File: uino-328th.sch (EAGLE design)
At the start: 11 parts, among them J1 USB_MICRO_B_2.0-TH

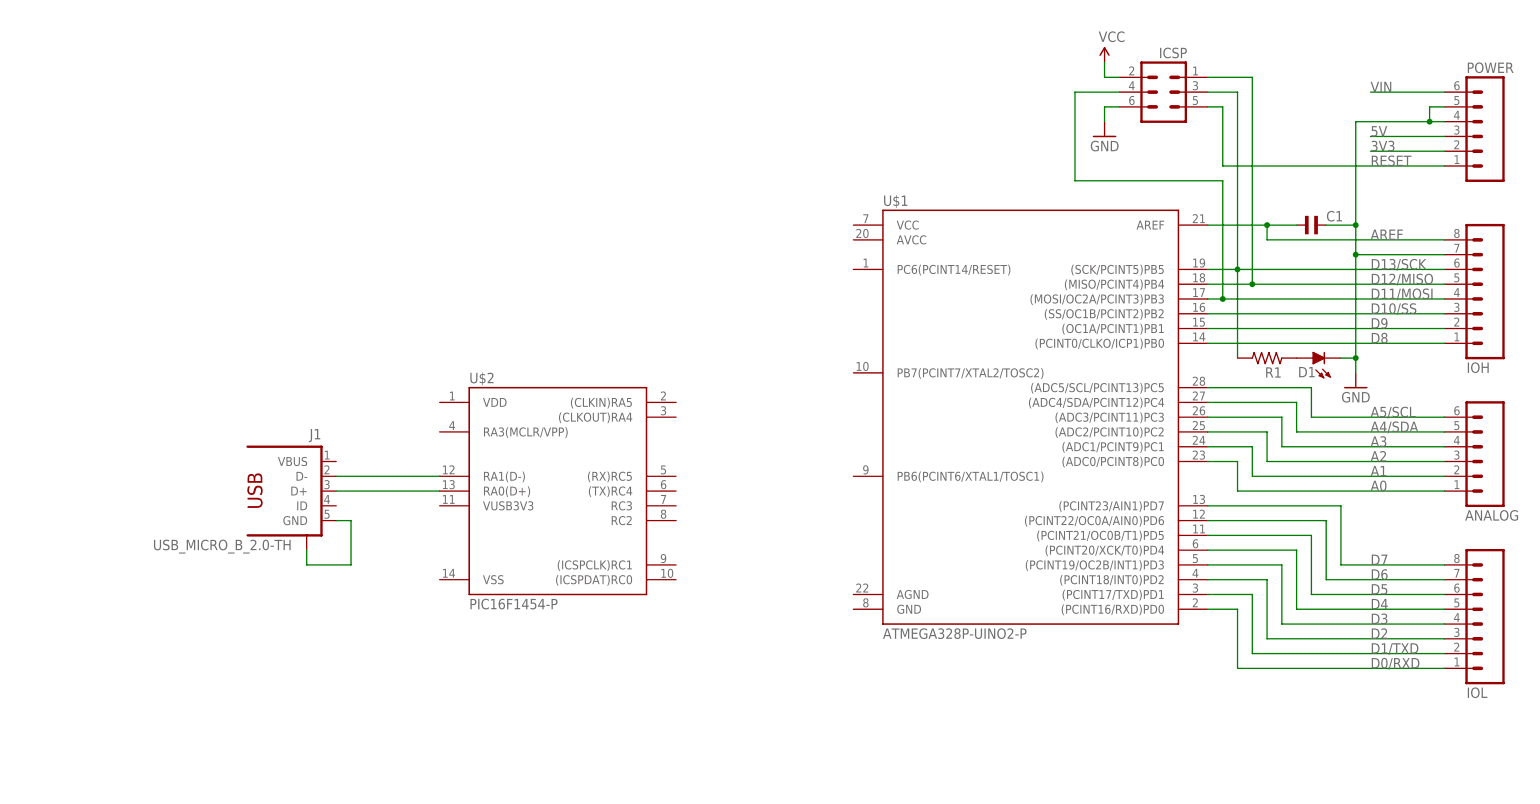
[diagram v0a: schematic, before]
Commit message: Schematic complete.
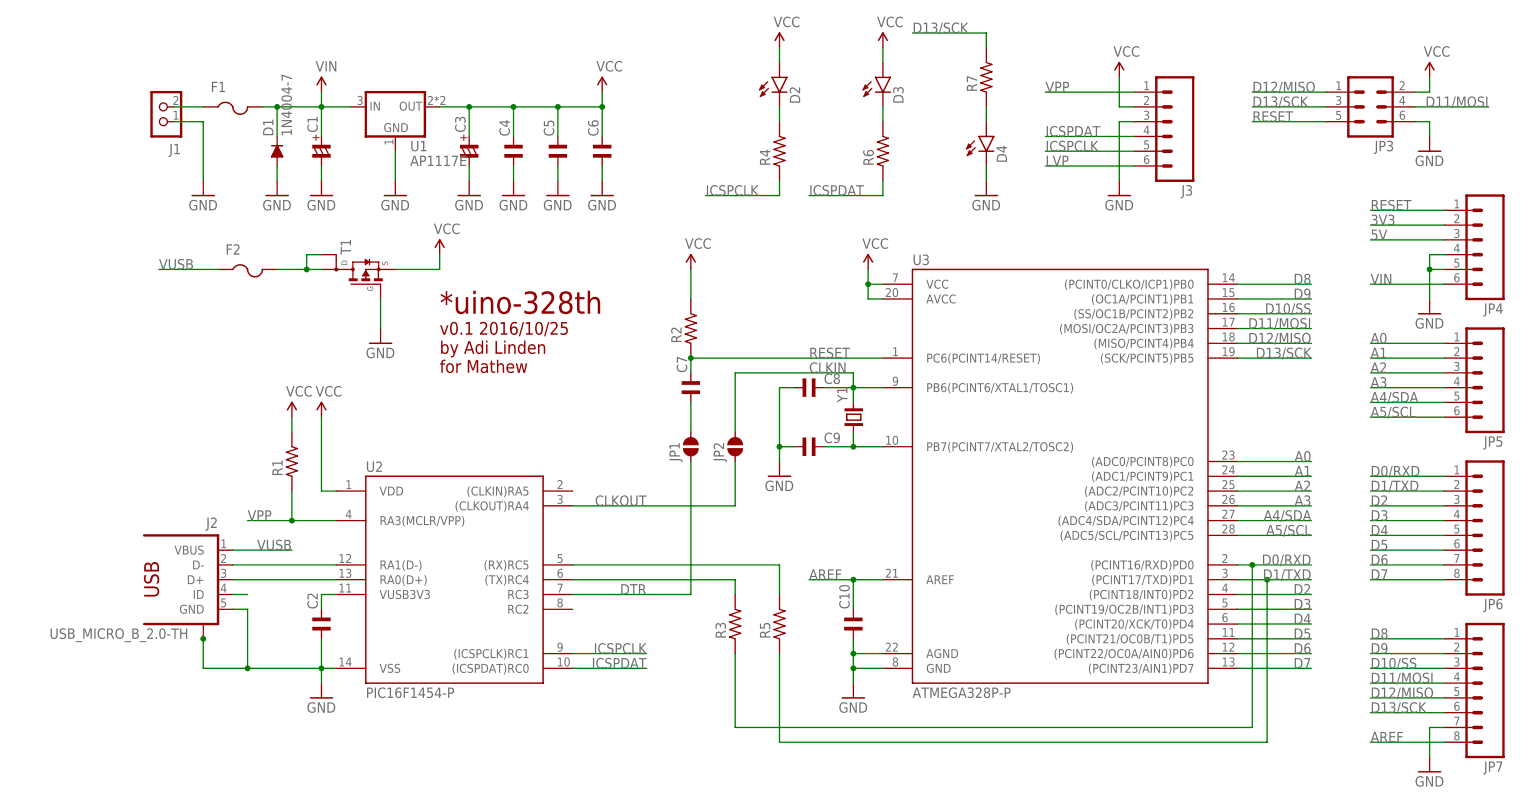
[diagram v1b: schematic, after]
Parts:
- removed ANALOG, POWER: (no value), SparkFun:M06SIP
- removed ICSP: M03X2, adilinden:M03X2
- removed IOH, IOL: (no value), SparkFun:M081X08
- removed U$1: ATMEGA328P-UINO2-P, adi-atmega:ATMEGA328P-UINO2-P
- removed U$2: PIC16F1454-P, adi-pic:PIC16F1454-P
- added C10, C2, C4, C5, C6, C7, C8, C9: (no value), rc-master-th:C_C025-040X018
- added C3: (no value), rc-master-th:CP_TT025-040
- added D2, D3, D4: (no value), SparkFun-LED:LED3MM
- added F1, F2: (no value), adi-misc:FUSE_PTC-1206
- added J2: USB_MICRO_B_2.0-TH, adi-misc:USB_MICRO_B_2.0-TH
- added J3: (no value), SparkFun-Connectors:M06LOCK
- added JP1, JP2: SJ-035, jumpers:SJ-035
- added JP3: M03X2, adi-misc:M03X2
- added JP4, JP5: (no value), SparkFun:M06SIP
- added JP6, JP7: (no value), SparkFun:M081X08
- added R2, R3, R4, R5, R6, R7: (no value), rc-master-th:R_038X018
- added T1: (no value), zetex:PMOSSOT223
- added U1: AP1117E, v-reg:AP1117E
- added U2: PIC16F1454-P, adi-pic:PIC16F1454-P
- added U3: ATMEGA328P-P, adi-atmega:ATMEGA328P-P
- added Y1: (no value), crystal:CRYTALHC49S
- C1: device rc-master-th:C_C025-040X018 -> rc-master-th:CP_TT025-040
- D1: value (none) -> 1N4004-7; device led:LED3MM -> diode:1N4004-7
- J1: value USB_MICRO_B_2.0-TH -> CON_TERMINAL_BLOCK_02-5MM; device adilinden:USB_MICRO_B_2.0-TH -> dp_devices.v6:CON_TERMINAL_BLOCK_02-5MM
- R1: device rc-master-th:R_X0204/7 -> rc-master-th:R_038X018
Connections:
- removed net VCC: ICSP.2
- new net CLKIN: C8.2, JP2.2, U3.PB6(PCINT6/XTAL1/TOSC1), Y1.2
- new net CLKOUT: JP2.1, U2.(CLKOUT)RA4
- new net DTR: JP1.1, U2.RC3
- new net ICSPCLK: J3.5, R4.1, U2.(ICSPCLK)RC1
- new net ICSPDAT: J3.4, R6.1, U2.(ICSPDAT)RC0
- new net LVP: J3.6
- new net N$10: R5.2, U2.(RX)RC5
- new net N$12: D2.C, R4.2
- new net N$13: D3.C, R6.2
- new net N$15: F2.2, T1.D, T1.D2
- new net N$5: D4.A, R7.1
- new net N$6: J2.ID
- new net N$7: C9.2, U3.PB7(PCINT7/XTAL2/TOSC2), Y1.1
- new net N$8: F1.1, J1.2
- new net N$9: R3.2, U2.(TX)RC4
- new net VPP: J3.1, R1.1, U2.RA3(MCLR/VPP)
- new net VUSB: F2.1, J2.VBUS
- net 3V3: now also JP4.2; no longer POWER.2
- net 5V: now also C3.+, C4.2, C5.2, C6.2, D2.A, D3.A, J3.2, JP3.2, JP4.3, R1.2, R2.2, T1.S, U1.OUT, U2.VDD, U3.AVCC, U3.VCC; no longer POWER.3
- net A0: now also JP5.1, U3.(ADC0/PCINT8)PC0; no longer ANALOG.1, U$1.(ADC0/PCINT8)PC0
- net A1: now also JP5.2, U3.(ADC1/PCINT9)PC1; no longer ANALOG.2, U$1.(ADC1/PCINT9)PC1
- net A2: now also JP5.3, U3.(ADC2/PCINT10)PC2; no longer ANALOG.3, U$1.(ADC2/PCINT10)PC2
- net A3: now also JP5.4, U3.(ADC3/PCINT11)PC3; no longer ANALOG.4, U$1.(ADC3/PCINT11)PC3
- net A4/SDA: now also JP5.5, U3.(ADC4/SDA/PCINT12)PC4; no longer ANALOG.5, U$1.(ADC4/SDA/PCINT12)PC4
- net A5/SCL: now also JP5.6, U3.(ADC5/SCL/PCINT13)PC5; no longer ANALOG.6, U$1.(ADC5/SCL/PCINT13)PC5
- net AREF: now also C10.2, JP7.8, U3.AREF; no longer C1.1, IOH.8, U$1.AREF
- net D0/RXD: now also JP6.1, R3.1, U3.(PCINT16/RXD)PD0; no longer IOL.1, U$1.(PCINT16/RXD)PD0
- net D1/TXD: now also JP6.2, R5.1, U3.(PCINT17/TXD)PD1; no longer IOL.2, U$1.(PCINT17/TXD)PD1
- net D10/SS: now also JP7.3, U3.(SS/OC1B/PCINT2)PB2; no longer IOH.3, U$1.(SS/OC1B/PCINT2)PB2
- net D11/MOSI: now also JP3.4, JP7.4, U3.(MOSI/OC2A/PCINT3)PB3; no longer ICSP.4, IOH.4, U$1.(MOSI/OC2A/PCINT3)PB3
- net D12/MISO: now also JP3.1, JP7.5, U3.(MISO/PCINT4)PB4; no longer ICSP.1, IOH.5, U$1.(MISO/PCINT4)PB4
- net D13/SCK: now also JP3.3, JP7.6, R7.2, U3.(SCK/PCINT5)PB5; no longer ICSP.3, IOH.6, R1.2, U$1.(SCK/PCINT5)PB5
- net D2: now also JP6.3, U3.(PCINT18/INT0)PD2; no longer IOL.3, U$1.(PCINT18/INT0)PD2
- net D3: now also JP6.4, U3.(PCINT19/OC2B/INT1)PD3; no longer IOL.4, U$1.(PCINT19/OC2B/INT1)PD3
- net D4: now also JP6.5, U3.(PCINT20/XCK/T0)PD4; no longer IOL.5, U$1.(PCINT20/XCK/T0)PD4
- net D5: now also JP6.6, U3.(PCINT21/OC0B/T1)PD5; no longer IOL.6, U$1.(PCINT21/OC0B/T1)PD5
- net D6: now also JP6.7, U3.(PCINT22/OC0A/AIN0)PD6; no longer IOL.7, U$1.(PCINT22/OC0A/AIN0)PD6
- net D7: now also JP6.8, U3.(PCINT23/AIN1)PD7; no longer IOL.8, U$1.(PCINT23/AIN1)PD7
- net D8: now also JP7.1, U3.(PCINT0/CLKO/ICP1)PB0; no longer IOH.1, U$1.(PCINT0/CLKO/ICP1)PB0
- net D9: now also JP7.2, U3.(OC1A/PCINT1)PB1; no longer IOH.2, U$1.(OC1A/PCINT1)PB1
- net GND: now also C1.-, C10.1, C2.1, C3.-, C4.1, C5.1, C6.1, C8.1, C9.1, D1.A, D4.C, J1.1, J2.GND, J2.S1, J2.S2, J3.3, JP3.6, JP4.4, JP4.5, JP7.7, T1.G, U1.GND, U2.VSS, U3.AGND, U3.GND; no longer C1.2, D1.C, ICSP.6, IOH.7, POWER.4, POWER.5
- net N$1: now also C2.2, U2.VUSB3V3; no longer J1.D-, U$2.RA1(D-)
- net N$2: now also C7.1, JP1.2; no longer J1.D+, U$2.RA0(D+)
- net N$3: now also J2.D-, U2.RA1(D-); no longer J1.GND, J1.S1
- net N$4: now also J2.D+, U2.RA0(D+); no longer D1.A, R1.1
- net RESET: now also C7.2, JP3.5, JP4.1, R2.1, U3.PC6(PCINT14/RESET); no longer ICSP.5, POWER.1
- net VIN: now also C1.+, D1.C, F1.2, JP4.6, U1.IN; no longer POWER.6
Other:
- note added: "*uino-328th"
- note added: "v0.1 2016/10/25 by Adi Linden for Mathew"
- moved on the sheet: R1
